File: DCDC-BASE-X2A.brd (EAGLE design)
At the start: 50 x 70 mm, 7 parts

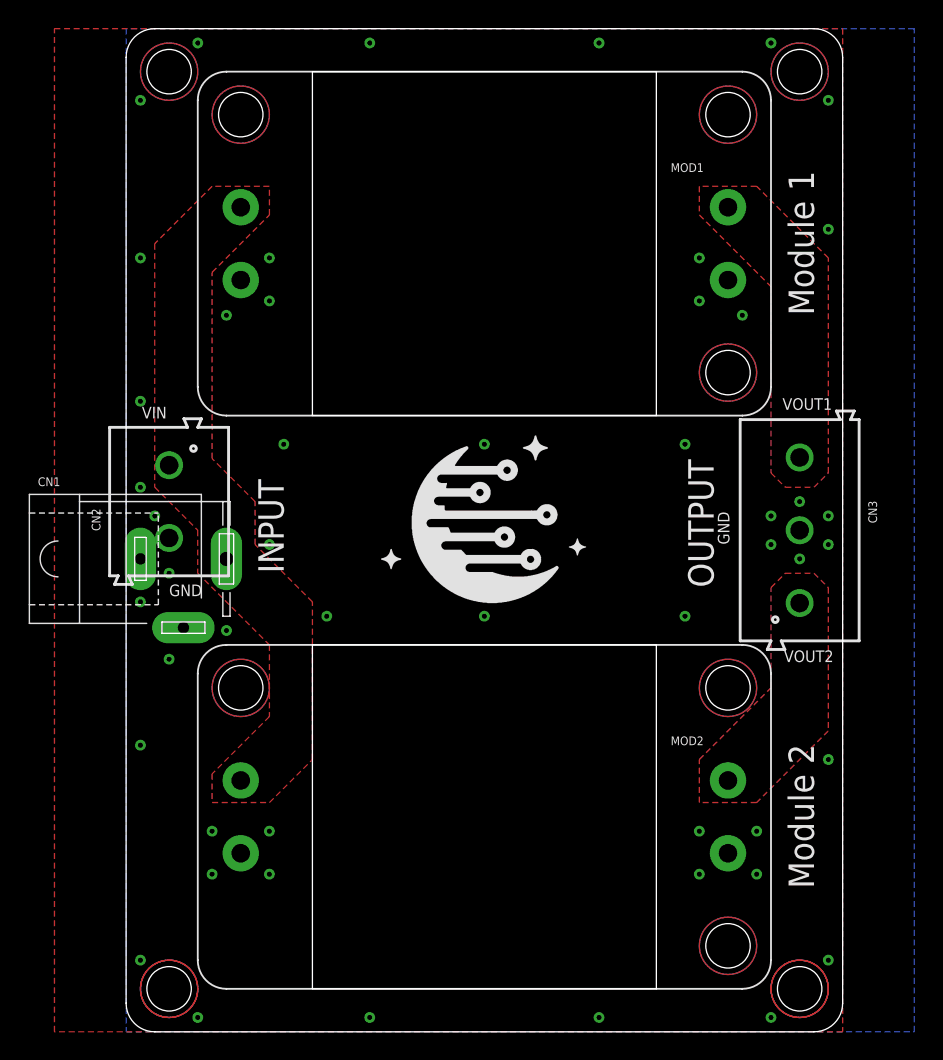
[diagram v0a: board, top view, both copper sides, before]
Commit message: Moved some stuff around on x2 boards. Generated CAM files. Generated PNG preview.
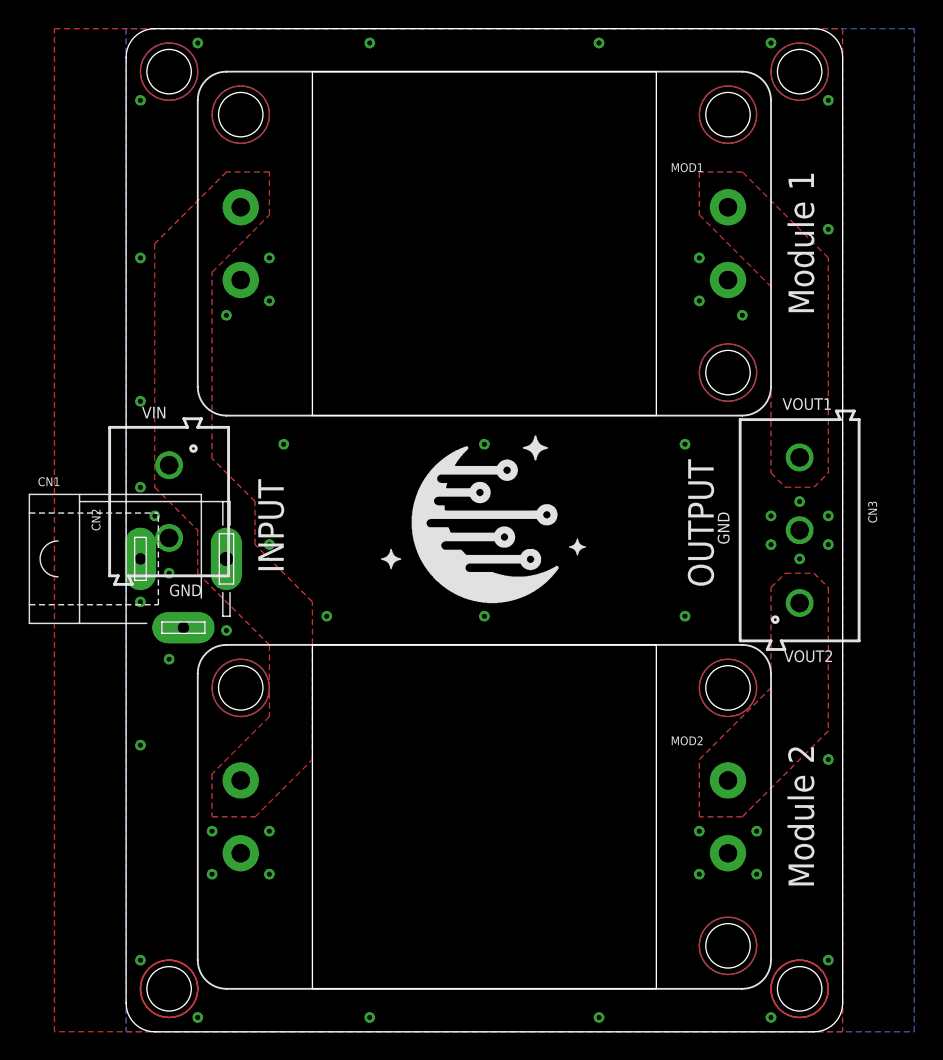
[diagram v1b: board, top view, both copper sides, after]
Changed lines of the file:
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@@
 <drawing>
 <settings>
-<setting alwaysvectorfont="yes"/>
+<setting alwaysvectorfont="no"/>
 <setting verticaltext="up"/>
 </settings>
@@
 <vertex x="10" y="22"/>
 <vertex x="6" y="18"/>
-<vertex x="6" y="16"/>
-<vertex x="10" y="16"/>
+<vertex x="6" y="15"/>
+<vertex x="9" y="15"/>
 <vertex x="13" y="19"/>
 <vertex x="13" y="30"/>
@@
 <vertex x="6" y="53"/>
 <vertex x="10" y="57"/>
-<vertex x="10" y="59"/>
-<vertex x="6" y="59"/>
+<vertex x="10" y="60"/>
+<vertex x="7" y="60"/>
 </polygon>
 </signal>
@@
 <contactref element="MOD1" pad="VOUT"/>
 <polygon width="0.3048" layer="1" thermals="no">
-<vertex x="40" y="59"/>
+<vertex x="40" y="60"/>
 <vertex x="40" y="57"/>
 <vertex x="45" y="52"/>
@@
 <vertex x="49" y="39"/>
 <vertex x="49" y="54"/>
-<vertex x="44" y="59"/>
+<vertex x="43" y="60"/>
 </polygon>
 </signal>
@@
 <contactref element="MOD2" pad="VOUT"/>
 <polygon width="0.3048" layer="1" thermals="no">
-<vertex x="40" y="16"/>
+<vertex x="40" y="15"/>
 <vertex x="40" y="19"/>
 <vertex x="45" y="24"/>
@@
 <vertex x="49" y="31"/>
 <vertex x="49" y="21"/>
-<vertex x="44" y="16"/>
+<vertex x="43" y="15"/>
 </polygon>
 </signal>
